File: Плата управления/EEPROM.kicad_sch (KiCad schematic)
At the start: 2 parts, among them U1 AT25xxx

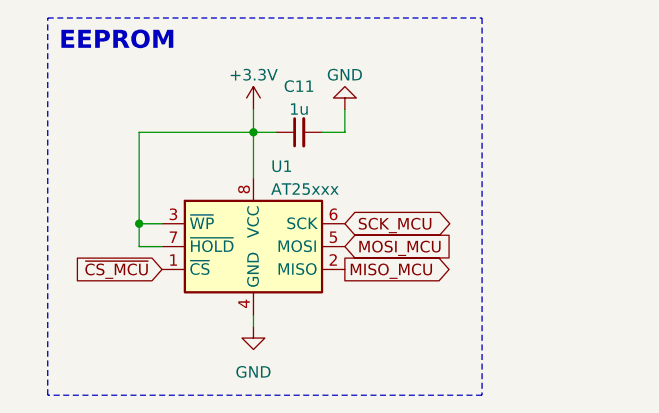
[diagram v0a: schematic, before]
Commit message: Редактировал схему
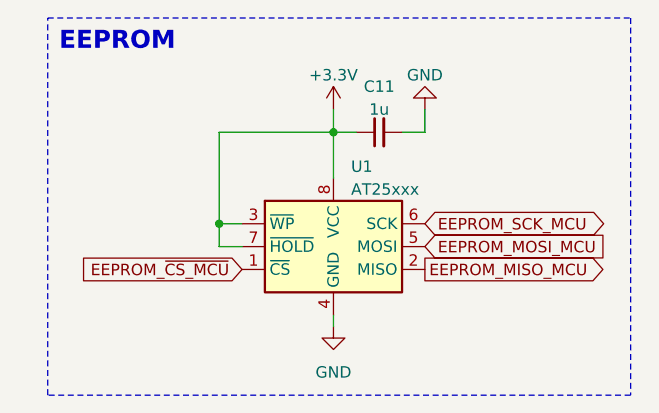
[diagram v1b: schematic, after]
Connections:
- net MISO_MCU renamed EEPROM_MISO_MCU
- net MOSI_MCU renamed EEPROM_MOSI_MCU
- net SCK_MCU renamed EEPROM_SCK_MCU
- net ~{CS_MCU} renamed EEPROM_~{CS_MCU}
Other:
- moved on the sheet: C11, U1
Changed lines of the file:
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@@
 (kicad_sch (version 20230121) (generator eeschema)
   (paper "A4")
-  (junction (at 25.4 38.1) (diameter 0) (color 0 0 0 0)
+  (junction (at 34.29 38.1) (diameter 0) (color 0 0 0 0)
   )
-  (junction (at 38.1 27.94) (diameter 0) (color 0 0 0 0)
+  (junction (at 46.99 27.94) (diameter 0) (color 0 0 0 0)
   )
-  (wire (pts (xy 38.1 33.02) (xy 38.1 27.94))
+  (wire (pts (xy 46.99 33.02) (xy 46.99 27.94))
     (stroke (width 0) (type default))
   )
-  (wire (pts (xy 25.4 27.94) (xy 38.1 27.94))
+  (wire (pts (xy 34.29 27.94) (xy 46.99 27.94))
     (stroke (width 0) (type default))
   )
-  (wire (pts (xy 38.1 27.94) (xy 40.64 27.94))
+  (wire (pts (xy 46.99 27.94) (xy 49.53 27.94))
     (stroke (width 0) (type default))
   )
-  (wire (pts (xy 38.1 25.4) (xy 38.1 27.94))
+  (wire (pts (xy 46.99 25.4) (xy 46.99 27.94))
     (stroke (width 0) (type default))
   )
-  (wire (pts (xy 45.72 27.94) (xy 48.26 27.94))
+  (wire (pts (xy 54.61 27.94) (xy 57.15 27.94))
     (stroke (width 0) (type default))
   )
-  (wire (pts (xy 25.4 40.64) (xy 25.4 38.1))
+  (wire (pts (xy 34.29 40.64) (xy 34.29 38.1))
     (stroke (width 0) (type default))
   )
-  (wire (pts (xy 27.94 40.64) (xy 25.4 40.64))
+  (wire (pts (xy 36.83 40.64) (xy 34.29 40.64))
     (stroke (width 0) (type default))
   )
-  (wire (pts (xy 25.4 38.1) (xy 27.94 38.1))
+  (wire (pts (xy 34.29 38.1) (xy 36.83 38.1))
     (stroke (width 0) (type default))
   )
-  (wire (pts (xy 25.4 38.1) (xy 25.4 27.94))
+  (wire (pts (xy 34.29 38.1) (xy 34.29 27.94))
     (stroke (width 0) (type default))
   )
-  (wire (pts (xy 38.1 48.26) (xy 38.1 49.53))
+  (wire (pts (xy 46.99 48.26) (xy 46.99 49.53))
     (stroke (width 0) (type default))
   )
-  (wire (pts (xy 48.26 27.94) (xy 48.26 25.4))
+  (wire (pts (xy 57.15 27.94) (xy 57.15 25.4))
     (stroke (width 0) (type default))
   )
-  (rectangle (start 15.24 15.24) (end 63.5 57.15)
+  (rectangle (start 15.24 15.24) (end 80.01 57.15)
     (stroke (width 0) (type dot))
     (fill (type none))
@@
     (effects (font (size 2 2) (thickness 0.4) bold) (justify left bottom))
   )
-  (global_label "MISO_MCU" (shape output) (at 48.26 43.18 0) (fields_autoplaced)
+  (global_label "EEPROM_MISO_MCU" (shape output) (at 57.15 43.18 0) (fields_autoplaced)
     (effects (font (size 1.27 1.27)) (justify left))
-    (property "Intersheetrefs" "${INTERSHEET_REFS}" (at 60.7815 43.18 0)
+    (property "Intersheetrefs" "${INTERSHEET_REFS}" (at 78.3384 43.18 0)
       (effects (font (size 1.27 1.27)) (justify left) hide)
     )
   )
-  (global_label "~{CS_MCU}" (shape input) (at 27.94 43.18 180) (fields_autoplaced)
+  (global_label "EEPROM_~{CS_MCU}" (shape input) (at 36.83 43.18 180) (fields_autoplaced)
     (effects (font (size 1.27 1.27)) (justify right))
-    (property "Intersheetrefs" "${INTERSHEET_REFS}" (at 17.5352 43.18 0)
+    (property "Intersheetrefs" "${INTERSHEET_REFS}" (at 17.7583 43.18 0)
       (effects (font (size 1.27 1.27)) (justify right) hide)
     )
   )
-  (global_label "SCK_MCU" (shape bidirectional) (at 48.26 38.1 0) (fields_autoplaced)
+  (global_label "EEPROM_SCK_MCU" (shape bidirectional) (at 57.15 38.1 0) (fields_autoplaced)
     (effects (font (size 1.27 1.27)) (justify left))
-    (property "Intersheetrefs" "${INTERSHEET_REFS}" (at 61.0461 38.1 0)
+    (property "Intersheetrefs" "${INTERSHEET_REFS}" (at 78.603 38.1 0)
       (effects (font (size 1.27 1.27)) (justify left) hide)
     )
   )
-  (global_label "MOSI_MCU" (shape input) (at 48.26 40.64 0) (fields_autoplaced)
+  (global_label "EEPROM_MOSI_MCU" (shape input) (at 57.15 40.64 0) (fields_autoplaced)
     (effects (font (size 1.27 1.27)) (justify left))
-    (property "Intersheetrefs" "${INTERSHEET_REFS}" (at 60.7815 40.64 0)
+    (property "Intersheetrefs" "${INTERSHEET_REFS}" (at 78.3384 40.64 0)
       (effects (font (size 1.27 1.27)) (justify left) hide)
     )
   )
-  (symbol (lib_id "Device:C_Small") (at 43.18 27.94 90) (unit 1)
+  (symbol (lib_id "Device:C_Small") (at 52.07 27.94 90) (unit 1)
     (in_bom yes) (on_board yes) (dnp no) (fields_autoplaced)
-    (property "Reference" "C11" (at 43.1863 22.86 90)
+    (property "Reference" "C11" (at 52.0763 22.86 90)
       (effects (font (size 1.27 1.27)))
     )
-    (property "Value" "1u" (at 43.1863 25.4 90)
+    (property "Value" "1u" (at 52.0763 25.4 90)
       (effects (font (size 1.27 1.27)))
     )
-    (property "Footprint" "Capacitor_SMD:C_0603_1608Metric_Pad1.08x0.95mm_HandSolder" (at 43.18 27.94 0)
+    (property "Footprint" "Capacitor_SMD:C_0603_1608Metric_Pad1.08x0.95mm_HandSolder" (at 52.07 27.94 0)
       (effects (font (size 1.27 1.27)) hide)
     )
-    (property "Datasheet" "~" (at 43.18 27.94 0)
+    (property "Datasheet" "~" (at 52.07 27.94 0)
       (effects (font (size 1.27 1.27)) hide)
     )
@@
     )
   )
-  (symbol (lib_id "power:GND") (at 38.1 49.53 0) (unit 1)
+  (symbol (lib_id "power:GND") (at 46.99 49.53 0) (unit 1)
     (in_bom yes) (on_board yes) (dnp no) (fields_autoplaced)
-    (property "Reference" "#PWR0108" (at 38.1 55.88 0)
+    (property "Reference" "#PWR0108" (at 46.99 55.88 0)
       (effects (font (size 1.27 1.27)) hide)
     )
-    (property "Value" "GND" (at 38.1 54.61 0)
+    (property "Value" "GND" (at 46.99 54.61 0)
       (effects (font (size 1.27 1.27)))
     )
-    (property "Footprint" "" (at 38.1 49.53 0)
+    (property "Footprint" "" (at 46.99 49.53 0)
       (effects (font (size 1.27 1.27)) hide)
     )
-    (property "Datasheet" "" (at 38.1 49.53 0)
+    (property "Datasheet" "" (at 46.99 49.53 0)
       (effects (font (size 1.27 1.27)) hide)
     )
@@
     )
   )
-  (symbol (lib_id "Memory_EEPROM:AT25xxx") (at 38.1 40.64 0) (unit 1)
+  (symbol (lib_id "Memory_EEPROM:AT25xxx") (at 46.99 40.64 0) (unit 1)
     (in_bom yes) (on_board yes) (dnp no) (fields_autoplaced)
-    (property "Reference" "U1" (at 40.0559 31.75 0)
+    (property "Reference" "U1" (at 48.9459 31.75 0)
       (effects (font (size 1.27 1.27)) (justify left))
     )
-    (property "Value" "AT25xxx" (at 40.0559 34.29 0)
+    (property "Value" "AT25xxx" (at 48.9459 34.29 0)
       (effects (font (size 1.27 1.27)) (justify left))
     )
-    (property "Footprint" "Package_SO:SOIC-8_3.9x4.9mm_P1.27mm" (at 38.1 40.64 0)
+    (property "Footprint" "Package_SO:SOIC-8_3.9x4.9mm_P1.27mm" (at 46.99 40.64 0)
       (effects (font (size 1.27 1.27)) hide)
     )
-    (property "Datasheet" "http://ww1.microchip.com/downloads/en/DeviceDoc/Atmel-8707-SEEPROM-AT25010B-020B-040B-Datasheet.pdf" (at 38.1 40.64 0)
+    (property "Datasheet" "http://ww1.microchip.com/downloads/en/DeviceDoc/Atmel-8707-SEEPROM-AT25010B-020B-040B-Datasheet.pdf" (at 46.99 40.64 0)
       (effects (font (size 1.27 1.27)) hide)
     )
@@
     )
   )
-  (symbol (lib_id "power:+3.3V") (at 38.1 25.4 0) (unit 1)
+  (symbol (lib_id "power:+3.3V") (at 46.99 25.4 0) (unit 1)
     (in_bom yes) (on_board yes) (dnp no) (fields_autoplaced)
-    (property "Reference" "#PWR0110" (at 38.1 29.21 0)
+    (property "Reference" "#PWR0110" (at 46.99 29.21 0)
       (effects (font (size 1.27 1.27)) hide)
     )
-    (property "Value" "+3.3V" (at 38.1 21.59 0)
+    (property "Value" "+3.3V" (at 46.99 21.59 0)
       (effects (font (size 1.27 1.27)))
     )
-    (property "Footprint" "" (at 38.1 25.4 0)
+    (property "Footprint" "" (at 46.99 25.4 0)
       (effects (font (size 1.27 1.27)) hide)
     )
-    (property "Datasheet" "" (at 38.1 25.4 0)
+    (property "Datasheet" "" (at 46.99 25.4 0)
       (effects (font (size 1.27 1.27)) hide)
     )
@@
     )
   )
-  (symbol (lib_id "power:GND") (at 48.26 25.4 180) (unit 1)
+  (symbol (lib_id "power:GND") (at 57.15 25.4 180) (unit 1)
     (in_bom yes) (on_board yes) (dnp no) (fields_autoplaced)
-    (property "Reference" "#PWR0109" (at 48.26 19.05 0)
+    (property "Reference" "#PWR0109" (at 57.15 19.05 0)
       (effects (font (size 1.27 1.27)) hide)
     )
-    (property "Value" "GND" (at 48.26 21.59 0)
+    (property "Value" "GND" (at 57.15 21.59 0)
       (effects (font (size 1.27 1.27)))
     )
-    (property "Footprint" "" (at 48.26 25.4 0)
+    (property "Footprint" "" (at 57.15 25.4 0)
       (effects (font (size 1.27 1.27)) hide)
     )
-    (property "Datasheet" "" (at 48.26 25.4 0)
+    (property "Datasheet" "" (at 57.15 25.4 0)
       (effects (font (size 1.27 1.27)) hide)
     )
